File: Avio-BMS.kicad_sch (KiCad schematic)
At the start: 3 parts, among them J3 5077CR-16SMC2-BK-TR

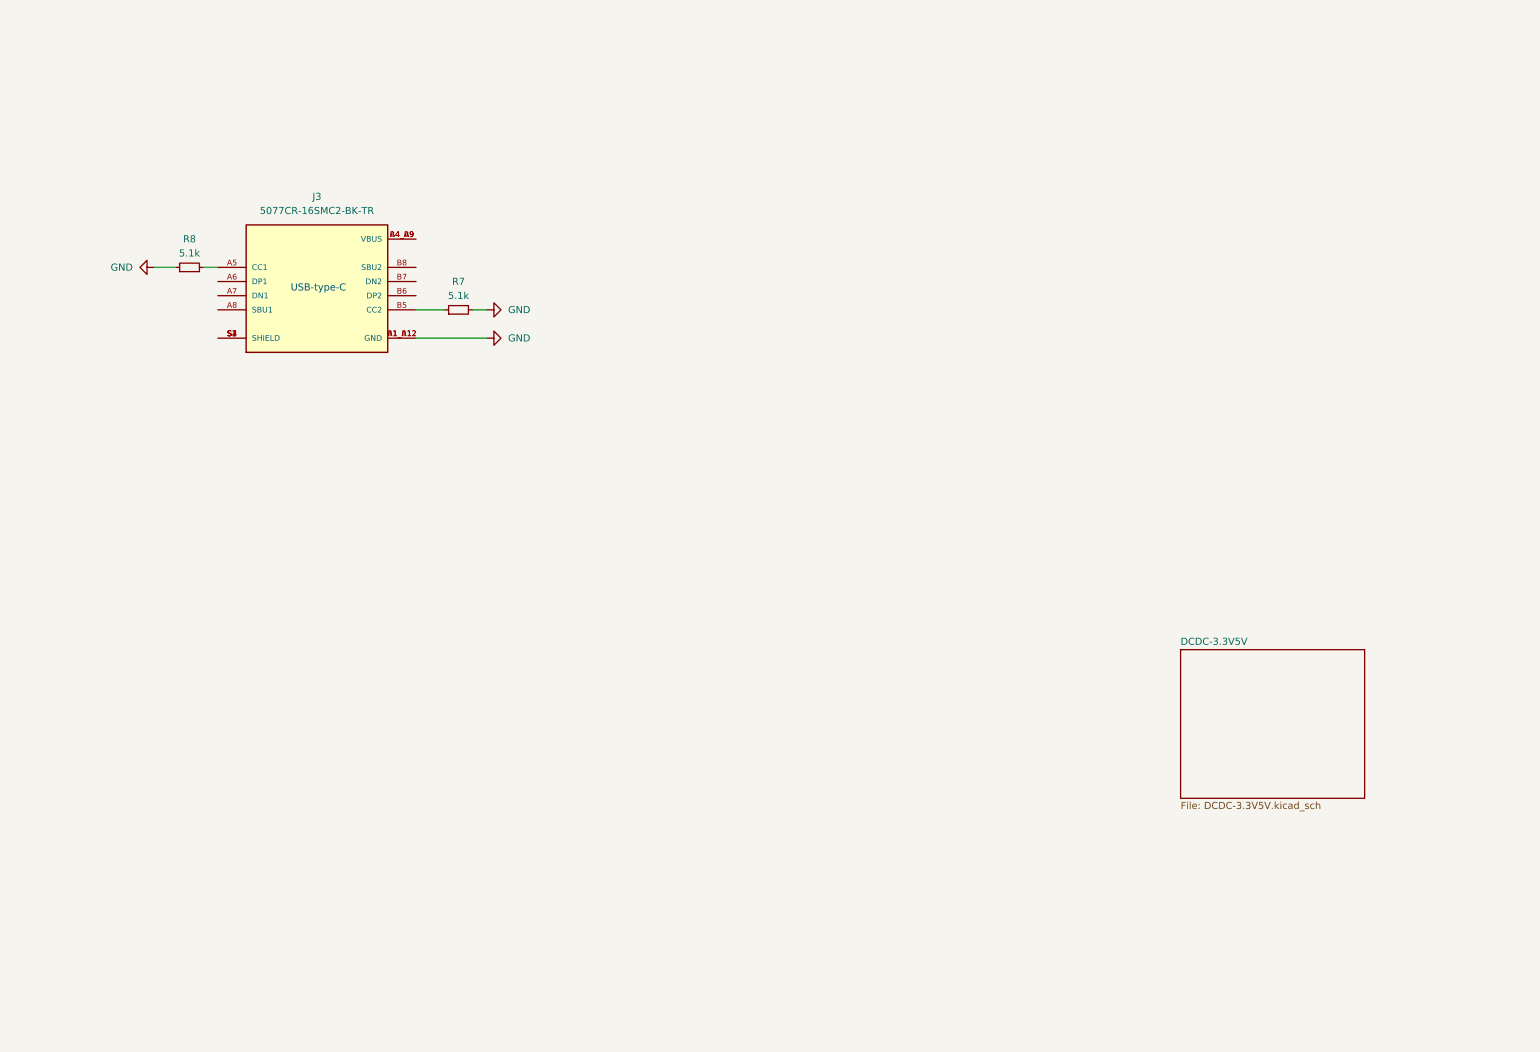
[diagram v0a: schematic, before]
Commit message: update
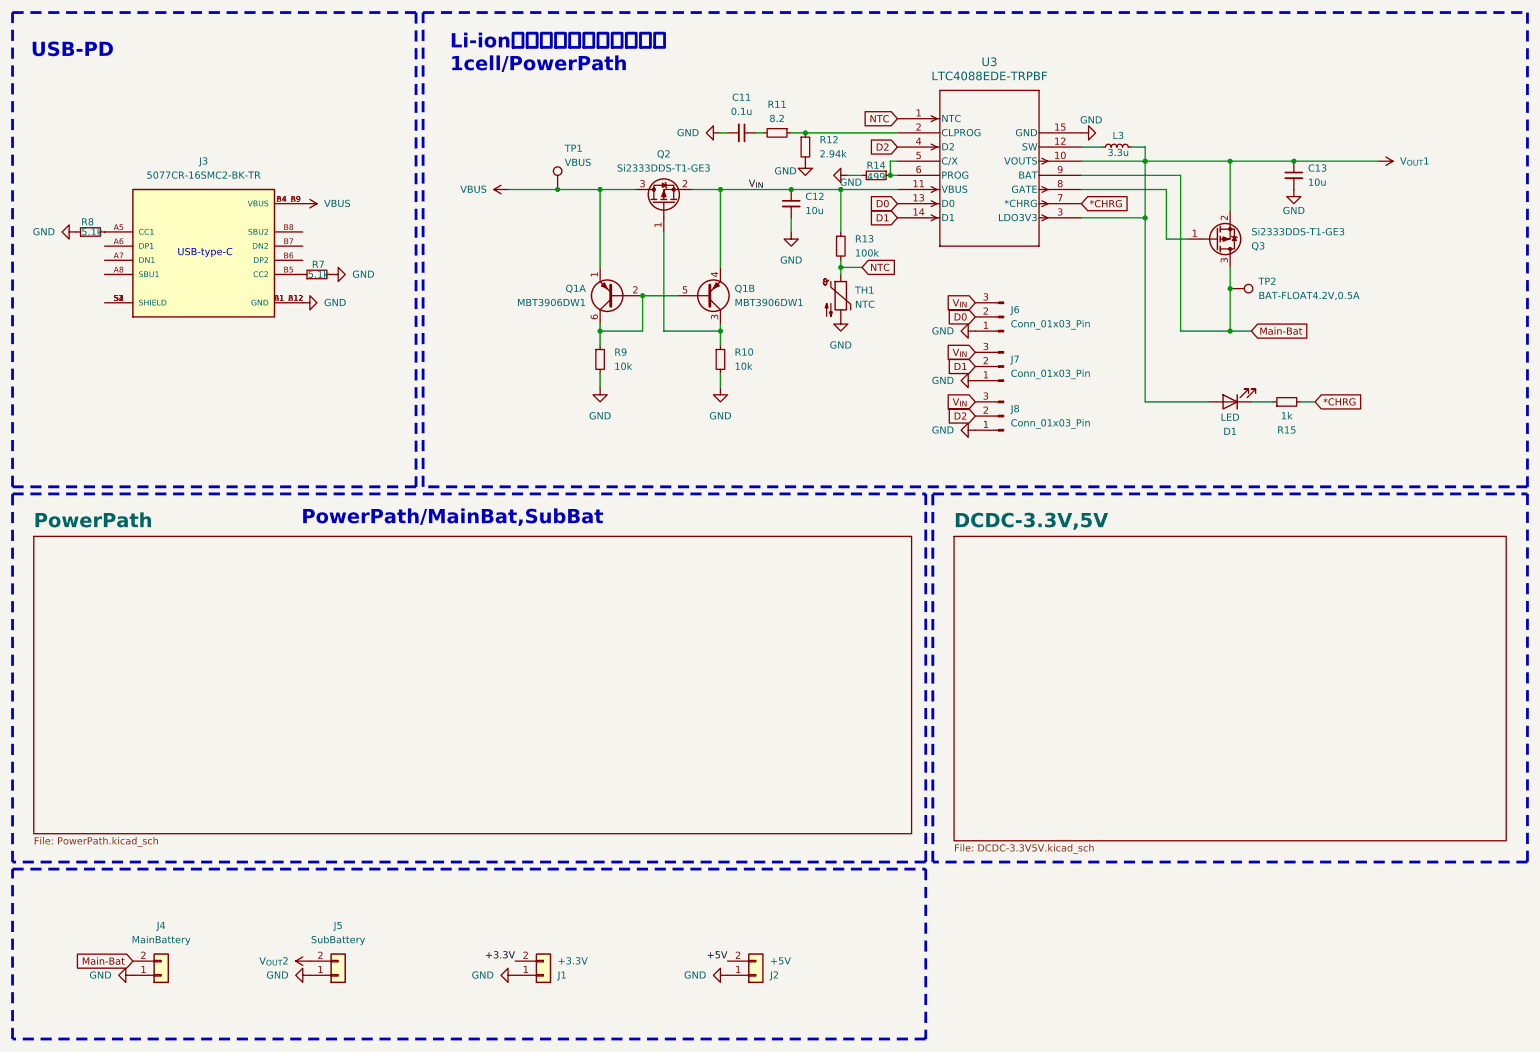
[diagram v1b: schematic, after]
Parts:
- added C11: 0.1u, Capacitor_SMD:C_0603_1608Metric_Pad1.08x0.95mm_HandSolder, symbol Device:C_Small
- added C12, C13: 10u, Capacitor_SMD:C_0805_2012Metric_Pad1.18x1.45mm_HandSolder, symbol Device:C_Small
- added D1: LED, LED_THT:LED_D4.0mm, symbol Device:LED
- added J1: +3.3V, Connector_JST:JST_XA_B02B-XASK-1_1x02_P2.50mm_Vertical, symbol Connector_Generic:Conn_01x02
- added J2: +5V, Connector_JST:JST_XA_B02B-XASK-1_1x02_P2.50mm_Vertical, symbol Connector_Generic:Conn_01x02
- added J4: MainBattery, Connector_JST:JST_XA_B02B-XASK-1_1x02_P2.50mm_Vertical, symbol Connector_Generic:Conn_01x02
- added J5: SubBattery, Connector_JST:JST_XA_B02B-XASK-1_1x02_P2.50mm_Vertical, symbol Connector_Generic:Conn_01x02
- added J6, J7, J8: Conn_01x03_Pin, Connector_PinHeader_2.54mm:PinHeader_1x03_P2.54mm_Vertical, symbol Connector:Conn_01x03_Pin
- added L3: 3.3u, symbol Device:L_Small
- added Q1: MBT3906DW1, Package_TO_SOT_SMD:SOT-363_SC-70-6, symbol Transistor_BJT:MBT3906DW1
- added Q2, Q3: Si2333DDS-T1-GE3, Package_TO_SOT_SMD:SOT-23-3, symbol Transistor_FET:Si2319CDS
- added R10, R9: 10k, Resistor_SMD:R_0603_1608Metric_Pad0.98x0.95mm_HandSolder, symbol Device:R_Small
- added R11: 8.2, Resistor_SMD:R_0603_1608Metric_Pad0.98x0.95mm_HandSolder, symbol Device:R_Small
- added R12: 2.94k, Resistor_SMD:R_0603_1608Metric_Pad0.98x0.95mm_HandSolder, symbol Device:R_Small
- added R13: 100k, Resistor_SMD:R_0603_1608Metric_Pad0.98x0.95mm_HandSolder, symbol Device:R_Small
- added R14: 499, Resistor_SMD:R_0603_1608Metric_Pad0.98x0.95mm_HandSolder, symbol Device:R_Small
- added R15: 1k, Resistor_SMD:R_0603_1608Metric_Pad0.98x0.95mm_HandSolder, symbol Device:R_Small
- added TH1: NTC, symbol Device:Thermistor_NTC
- added TP1: VBUS, Connector_Pin:Pin_D1.1mm_L8.5mm_W2.5mm_FlatFork, symbol Connector:TestPoint
- added TP2: BAT-FLOAT4.2V,0.5A, Connector_Pin:Pin_D1.1mm_L8.5mm_W2.5mm_FlatFork, symbol Connector:TestPoint
- added U3: LTC4088EDE-TRPBF, footprints:DFN-14_DE_LIT, symbol 2024-10-02_05-23-37:LTC4088EDE-TRPBF
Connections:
- net GND: now also C11.2, C12.2, C13.2, J1.1 (Pin_1), J2.1 (Pin_1), J4.1 (Pin_1), J5.1 (Pin_1), J6.1 (Pin_1), J7.1 (Pin_1), J8.1 (Pin_1), R10.2, R12.2, R14.2, R9.2, TH1.2, U3.15 (GND)
- net VBUS: now reaches J3.A4_B9 (VBUS), J3.B4_A9 (VBUS)
- net VBUS: now also Q1.1 (E1), Q2.3 (D), TP1.1
- new net: Q1.3 (C2), Q2.1 (G), R10.1
- new net: Q3.1 (G), U3.8 (GATE)
- new net: R11.1, R12.1, U3.2 (CLPROG)
- new net: C11.1, R11.2
- new net: D1.1 (K), R15.1
- new net: Q1.2 (B1), Q1.5 (B2), Q1.6 (C1), R9.1
- new net: L3.1, U3.12 (SW)
- new net: R14.1, U3.5 (C/X), U3.6 (PROG)
- new net *CHRG: R15.2, U3.7 (*CHRG)
- new net +3.3V: J1.2 (Pin_2)
- new net +5V: J2.2 (Pin_2)
- new net D0: J6.2 (Pin_2), U3.13 (D0)
- new net D1: J7.2 (Pin_2), U3.14 (D1)
- new net D2: J8.2 (Pin_2), U3.4 (D2)
- new net Main-Bat: J4.2 (Pin_2), Q3.3 (D), TP2.1, U3.9 (BAT)
- new net NTC: R13.2, TH1.1, U3.1 (NTC)
- new net V_{IN}: C12.1, J6.3 (Pin_3), J7.3 (Pin_3), J8.3 (Pin_3), Q1.4 (E2), Q2.2 (S), R13.1, U3.11 (VBUS)
- new net V_{OUT}1: C13.1, D1.2 (A), L3.2, Q3.2 (S), U3.10 (VOUTS), U3.3 (LDO3V3)
- new net V_{OUT}2: J5.2 (Pin_2)
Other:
- sheet DCDC-3.3V5V renamed DCDC-3.3V,5V
- added sheet PowerPath (PowerPath.kicad_sch)
- note added: "Li-ionバッテリーチャージャー 1cell/PowerPath"
- note added: "PowerPath/MainBat,SubBat"
- note added: "USB-PD"
- moved on the sheet: J3, R7, R8

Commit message: Update KiCad project files
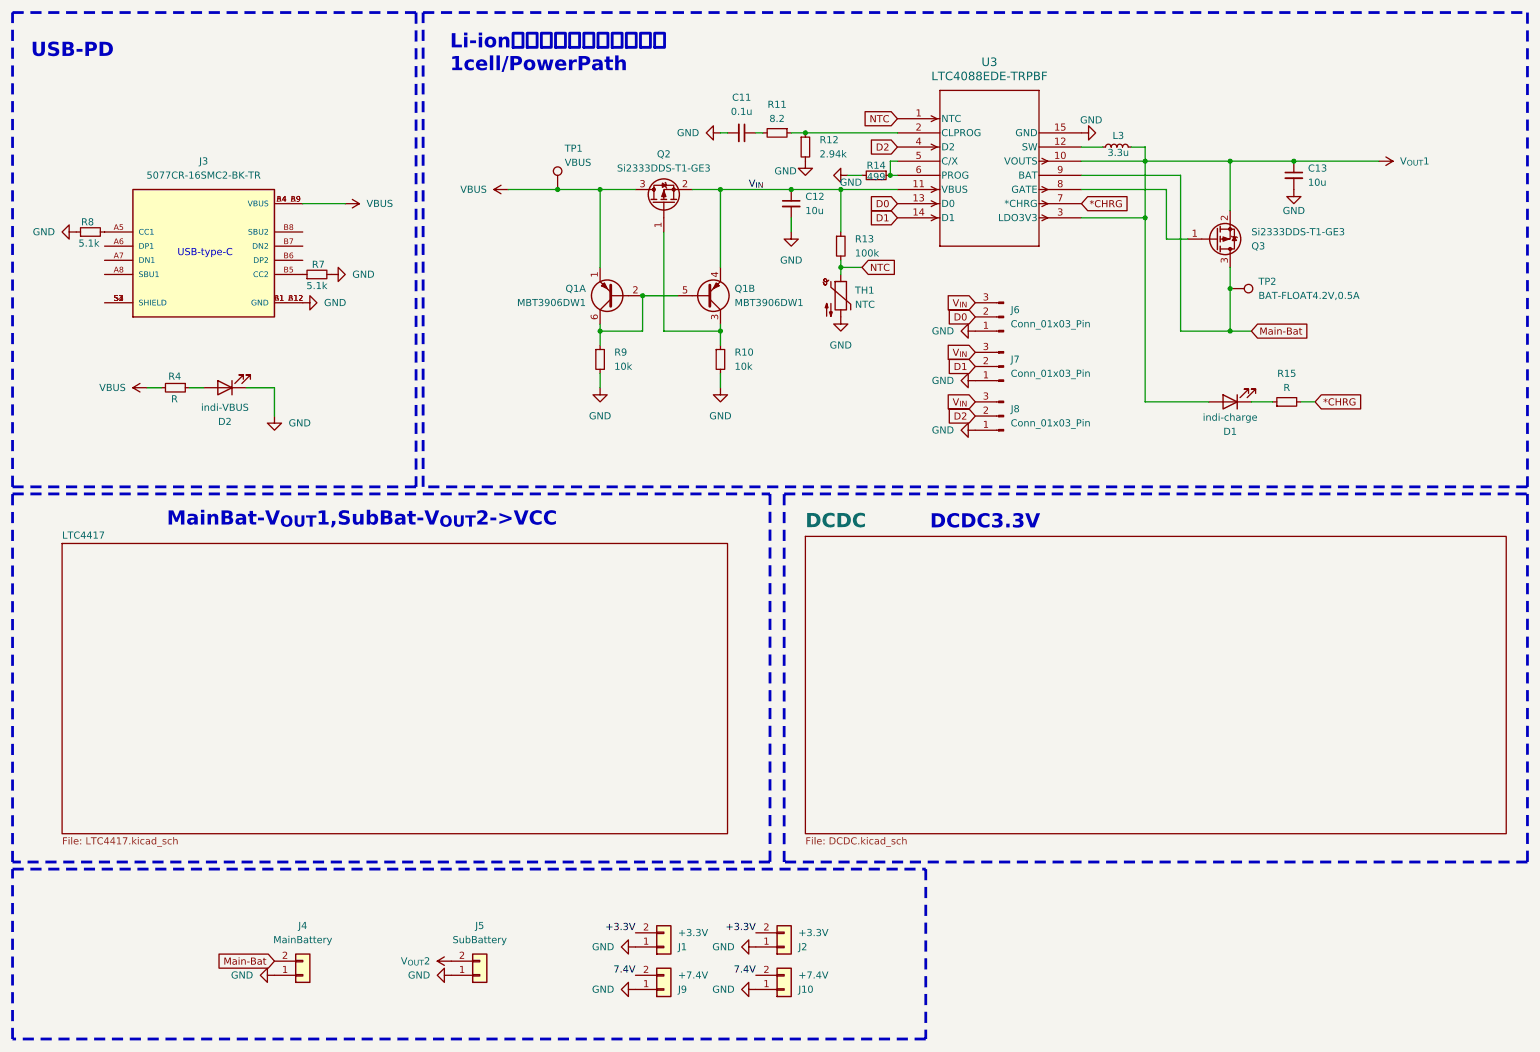
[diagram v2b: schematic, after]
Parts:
- added D2: indi-VBUS, LED_SMD:LED_0603_1608Metric, symbol Device:LED
- added J10, J9: +7.4V, Connector_JST:JST_XA_B02B-XASK-1_1x02_P2.50mm_Vertical, symbol Connector_Generic:Conn_01x02
- added R4: R, Resistor_SMD:R_0603_1608Metric_Pad0.98x0.95mm_HandSolder, symbol Device:R_Small
- D1: value LED -> indi-charge; footprint LED_THT:LED_D4.0mm -> LED_SMD:LED_0603_1608Metric
- J2: value +5V -> +3.3V
- R15: value 1k -> R
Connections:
- net +5V is gone; now on net +3.3V: J2.2 (Pin_2)
- net GND: now also D2.1 (K), J10.1 (Pin_1), J9.1 (Pin_1)
- net VBUS: now also R4.2
- new net: D2.2 (A), R4.1
- new net 7.4V: J10.2 (Pin_2), J9.2 (Pin_2)
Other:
- removed sheet DCDC-3.3V,5V
- removed sheet PowerPath
- added sheet DCDC (DCDC.kicad_sch)
- added sheet LTC4417 (LTC4417.kicad_sch)
- note added: "DCDC3.3V"
- note added: "MainBat-V_{OUT}1,SubBat-V_{OUT}2->VCC"
- note removed: "PowerPath/MainBat,SubBat"
- moved on the sheet: J1, J4, J5
